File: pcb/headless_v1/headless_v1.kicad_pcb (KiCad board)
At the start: 2 copper layers, 69 x 51 mm, 23 parts, among them J1 RJ10, J2 RJ10, J3 RJ10, J4 RJ10, J5 RJ10, J6 RJ10, J7 RJ10, J8 RJ10, SW1 RESET, U1 ProMicro

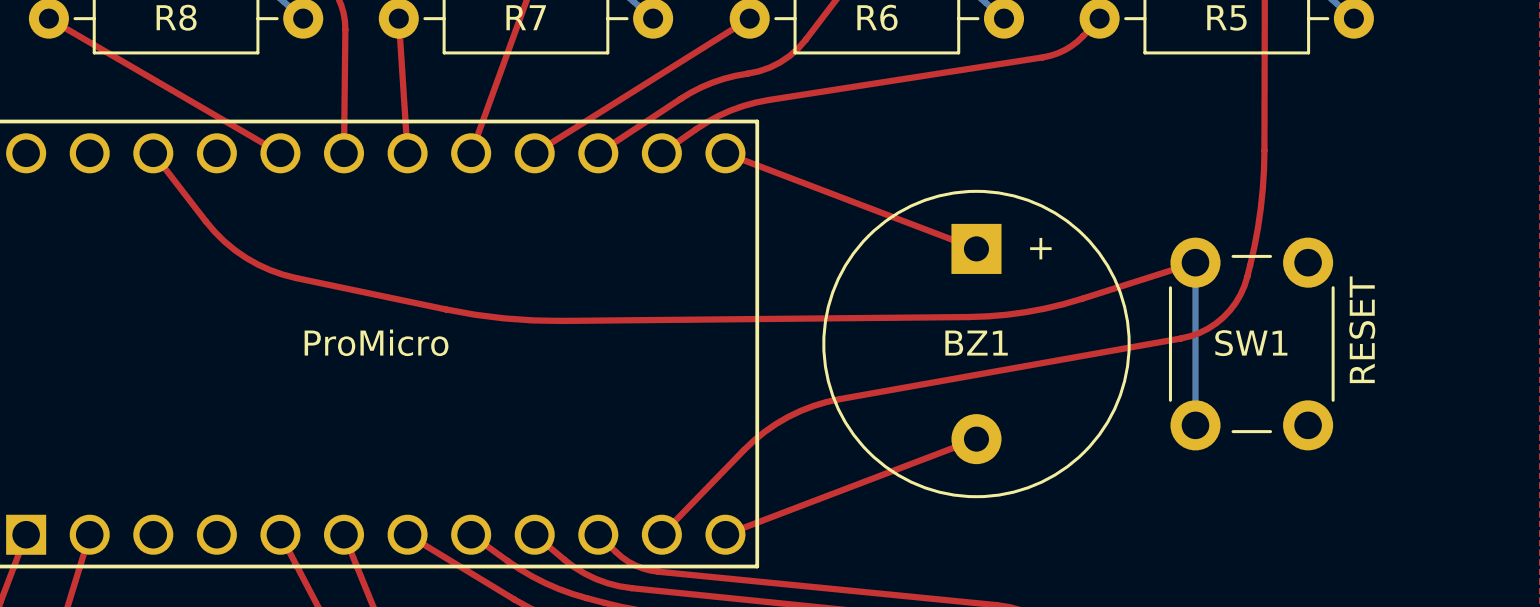
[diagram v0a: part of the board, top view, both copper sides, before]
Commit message: Headless PCB v1.2
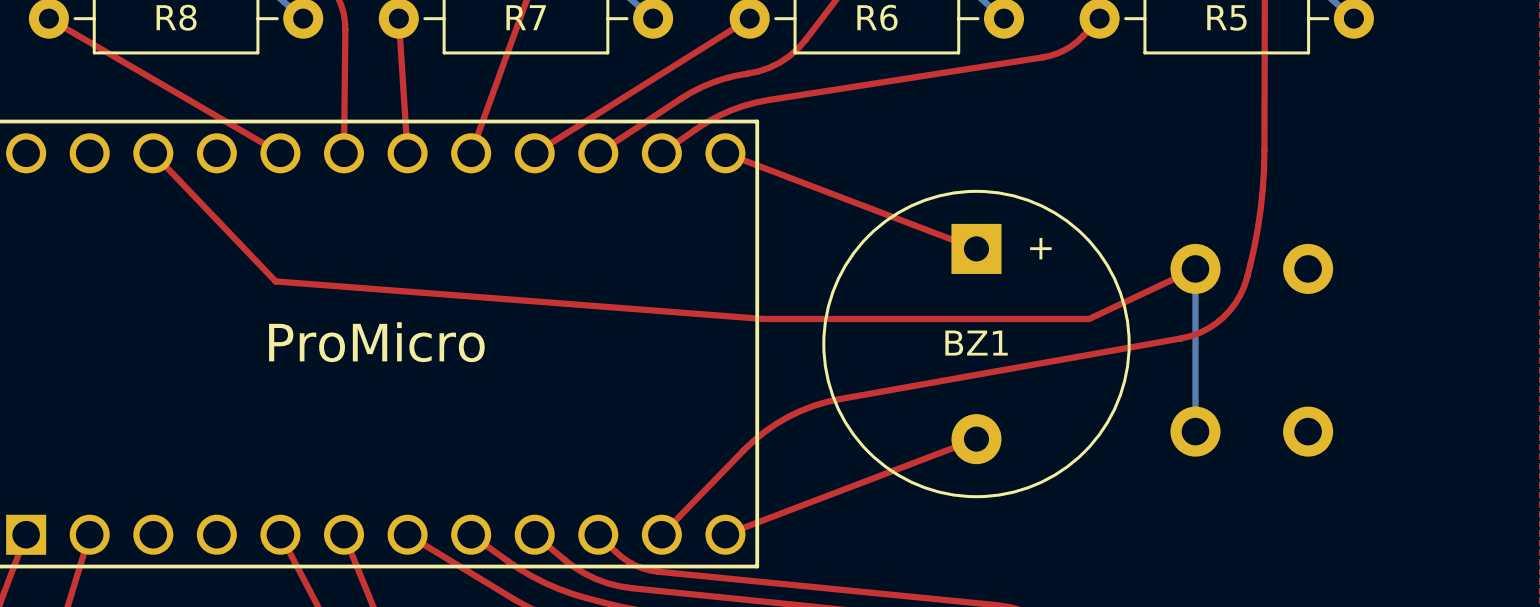
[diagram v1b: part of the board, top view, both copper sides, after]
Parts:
- SW1: moved to B.Cu
- moved SW1 6.25 mm to (98.8, 72.0), turned to -90 degrees
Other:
- board text added: "Headless Kamaji v1.2 Ilya Strukov 2022 github.com/iley/kamaji"
- board text removed: "Headless Kamaji v1.1 Ilya Strukov 2022 github.com/iley/kamaji"
